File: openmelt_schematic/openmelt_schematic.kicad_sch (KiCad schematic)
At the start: 11 parts, among them M1 Motor_DC, U1 A000053

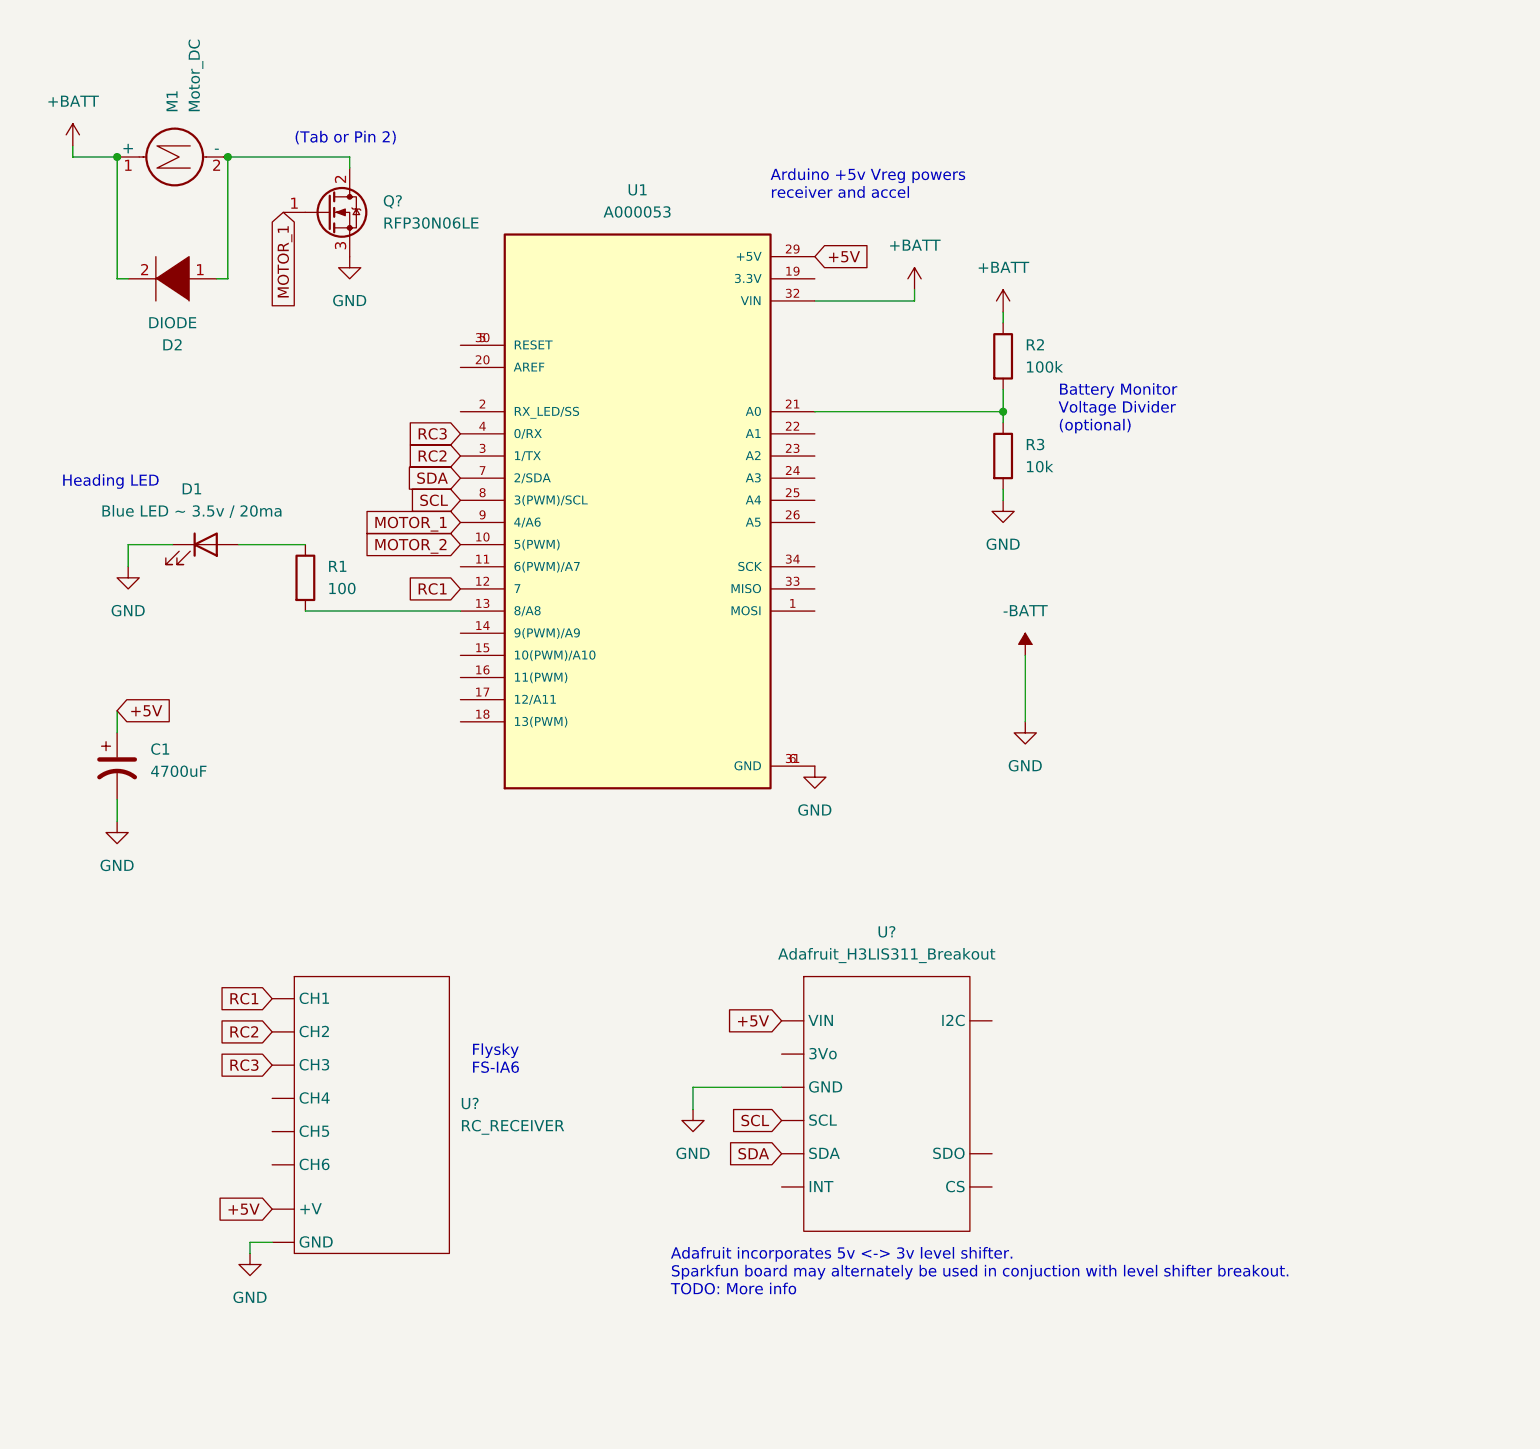
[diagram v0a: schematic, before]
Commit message: documentaion
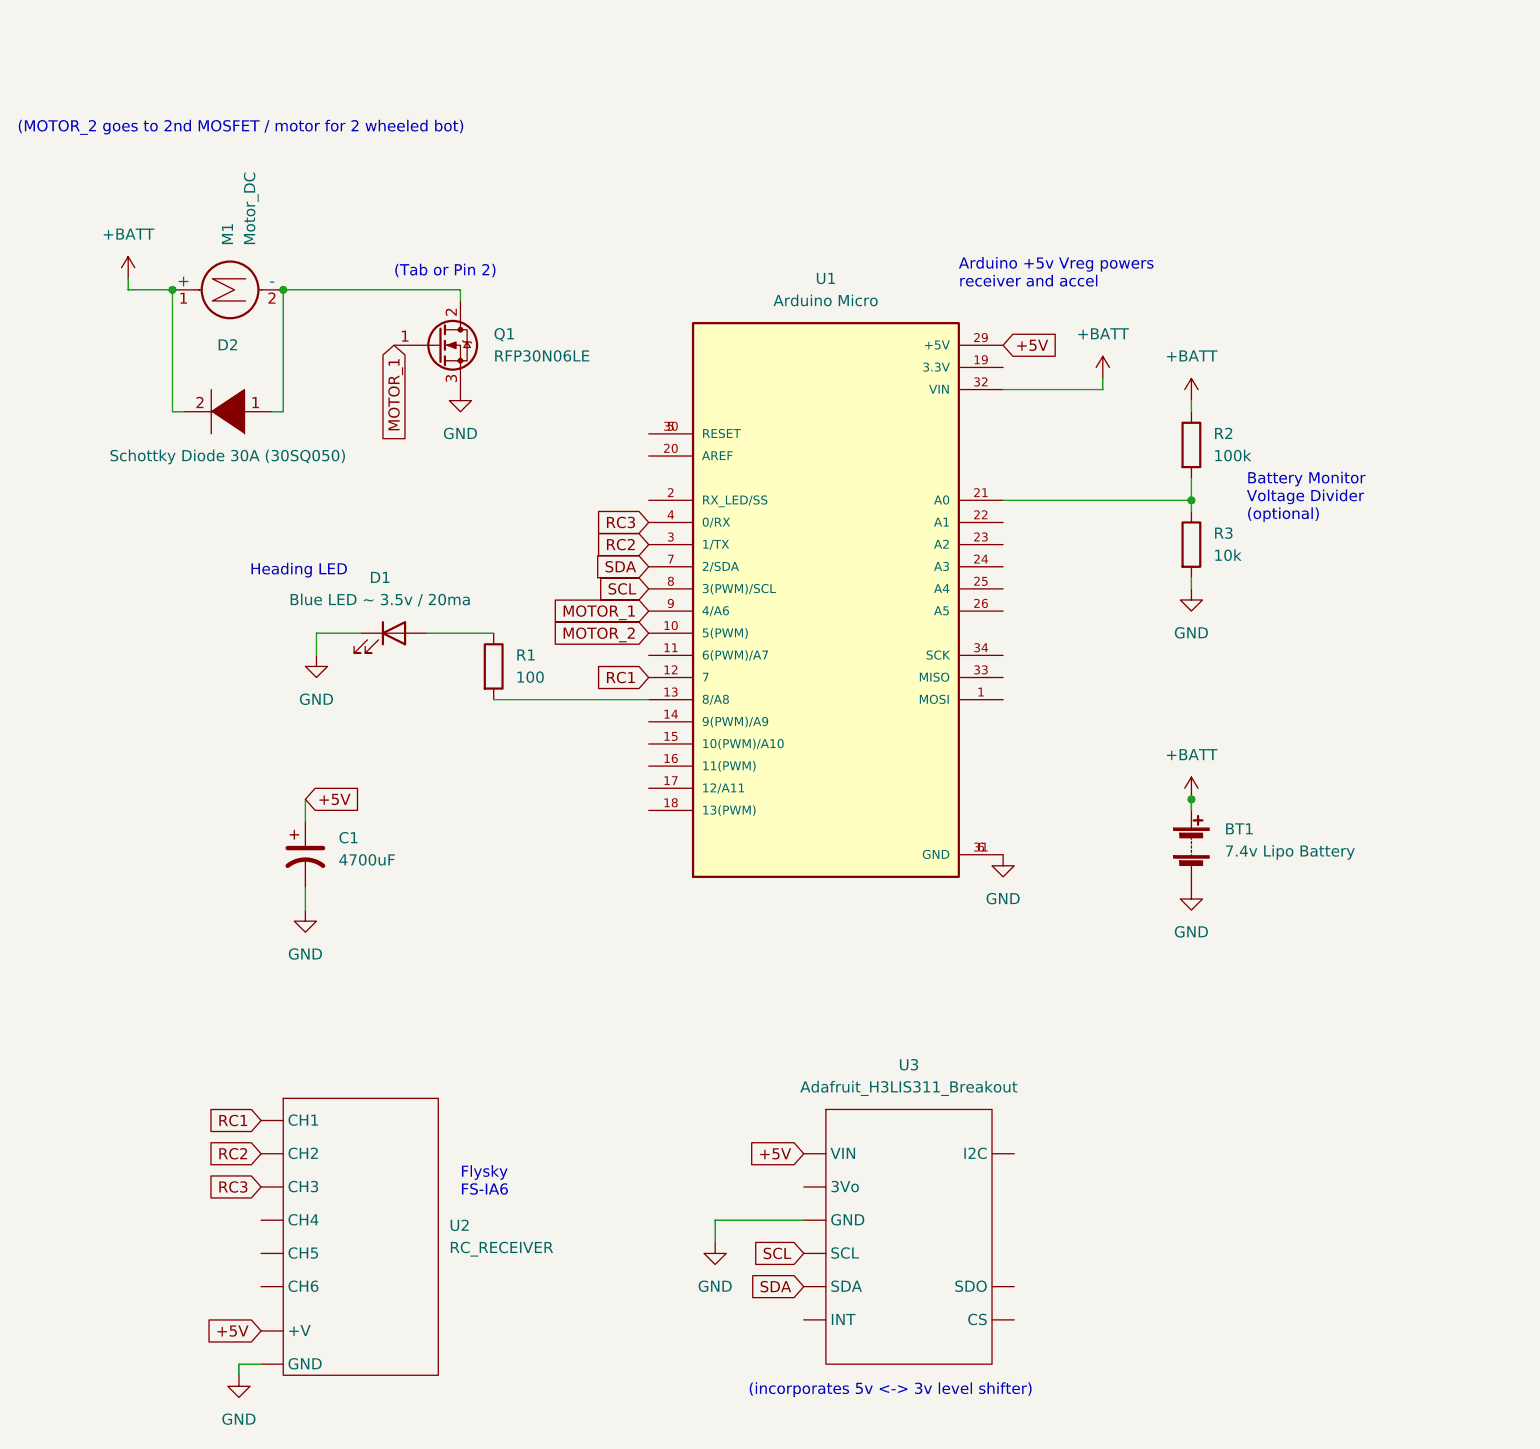
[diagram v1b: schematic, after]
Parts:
- added BT1: 7.4v Lipo Battery, symbol Device:Battery
- D2: value DIODE -> Schottky Diode 30A (30SQ050)
- U1: value A000053 -> Arduino Micro
- gave numbers to parts that had none: 3
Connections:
- net +BATT: now also BT1.1 (+)
- net -BATT renamed GND
- net GND: now also BT1.2 (-)
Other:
- note added: "(MOTOR_2 goes to 2nd MOSFET / motor for 2 wheeled bot)"
- note added: "(incorporates 5v <-> 3v level shifter)"
- note removed: "Adafruit incorporates 5v <-> 3v level shifter. Sparkfun board may alternately be used in conjuction with level shifter breakout. TODO: More info"
- moved on the sheet: C1, D1, D2, M1, Q1, R1, R2, R3, U1, U2, U3
